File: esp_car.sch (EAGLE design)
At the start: 50 parts, among them IC2 LT1963ES8-3.3, SW2 SK-12D01, U1 ESP-WROOM-32_NOFLASH

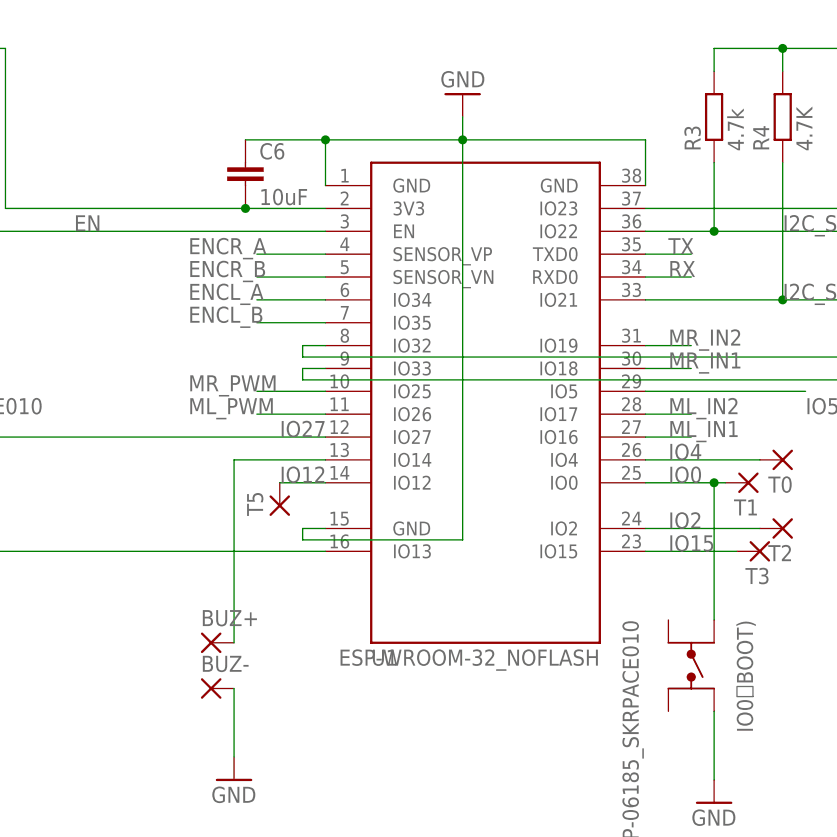
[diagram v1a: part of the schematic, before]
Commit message: wire 100% 初版
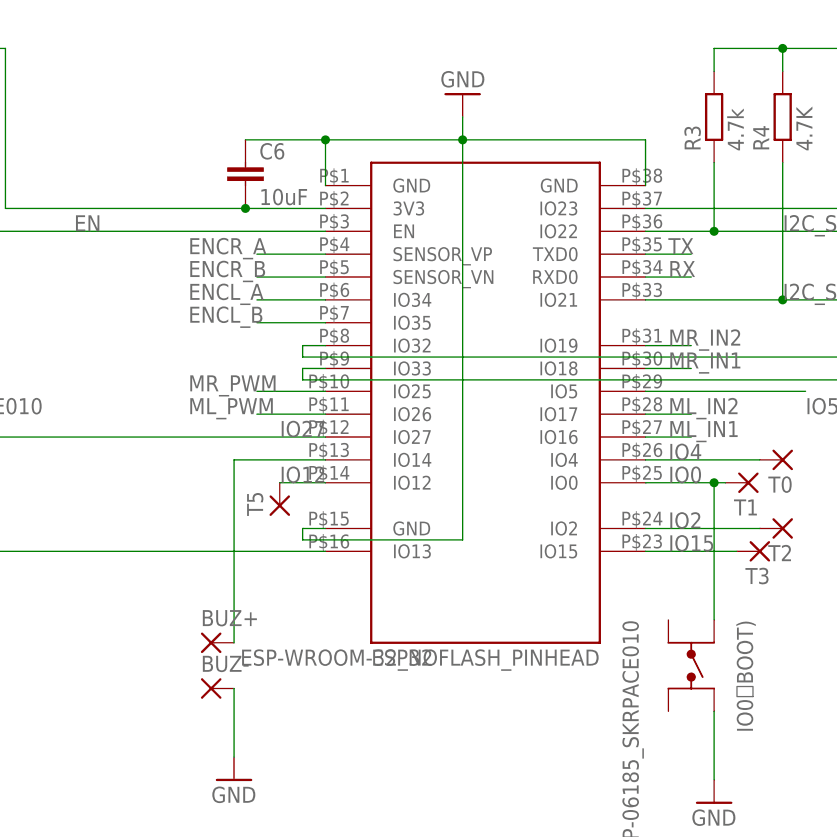
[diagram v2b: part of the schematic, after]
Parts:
- removed U1: ESP-WROOM-32_NOFLASH, esp32 _my:ESP-WROOM-32_NOFLASH
- added ESP32: ESP-WROOM-32_NOFLASH_PINHEAD, esp32 _my:ESP-WROOM-32_NOFLASH_PINHEAD
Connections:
- net +3V3: now also ESP32.3V3; no longer U1.3V3
- net EN: now also ESP32.EN; no longer U1.EN
- net ENCL_A: now also ESP32.IO34; no longer U1.IO34
- net ENCL_B: now also ESP32.IO35; no longer U1.IO35
- net ENCR_A: now also ESP32.SENSOR_VP; no longer U1.SENSOR_VP
- net ENCR_B: now also ESP32.SENSOR_VN; no longer U1.SENSOR_VN
- net GND: now also ESP32.GND@1, ESP32.GND@2, ESP32.GND@3; no longer U1.GND@1, U1.GND@2, U1.GND@3
- net I2C_SCL: now also ESP32.IO22; no longer U1.IO22
- net I2C_SDA: now also ESP32.IO21; no longer U1.IO21
- net IO0: now also ESP32.IO0; no longer U1.IO0
- net IO12: now also ESP32.IO12; no longer U1.IO12
- net IO15: now also ESP32.IO15; no longer U1.IO15
- net IO2: now also ESP32.IO2; no longer U1.IO2
- net IO27: now also ESP32.IO27; no longer U1.IO27
- net IO4: now also ESP32.IO4; no longer U1.IO4
- net IO5: now also ESP32.IO5; no longer U1.IO5
- net ML_IN1: now also ESP32.IO16; no longer U1.IO16
- net ML_IN2: now also ESP32.IO17; no longer U1.IO17
- net ML_PWM: now also ESP32.IO26; no longer U1.IO26
- net MR_IN1: now also ESP32.IO18; no longer U1.IO18
- net MR_IN2: now also ESP32.IO19; no longer U1.IO19
- net MR_PWM: now also ESP32.IO25; no longer U1.IO25
- net N$18: now also ESP32.IO13; no longer U1.IO13
- net N$19: now also ESP32.IO33; no longer U1.IO33
- net N$3: now also ESP32.IO32; no longer U1.IO32
- net N$5: now also ESP32.IO23; no longer U1.IO23
- net N$8: now also ESP32.IO14; no longer U1.IO14
- net RX: now also ESP32.RXD0; no longer U1.RXD0
- net TX: now also ESP32.TXD0; no longer U1.TXD0
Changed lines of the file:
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@@
 <?xml version="1.0" encoding="utf-8"?>
 <!DOCTYPE eagle SYSTEM "eagle.dtd">
-<eagle version="9.0.0">
+<eagle version="9.0.1">
 <drawing>
 <settings>
@@
 <clearance class="0" value="0.1524"/>
 </class>
-<class number="1" name="L" width="1.016" drill="0.4064">
+<class number="1" name="L" width="1.016" drill="0.8128">
 <clearance class="1" value="0.1524"/>
 </class>
@@
 <part name="GY-530C" library="pinhead" deviceset="PINHD-1X5" device=""/>
 <part name="GY-530L" library="pinhead" deviceset="PINHD-1X5" device=""/>
-<part name="U1" library="esp32 _my" deviceset="ESP-WROOM-32_NOFLASH" device=""/>
 <part name="U$1" library="adafruit_my" deviceset="TB6612_NEW" device=""/>
+<part name="ESP32" library="esp32 _my" deviceset="ESP-WROOM-32_NOFLASH_PINHEAD" device=""/>
 </parts>
 <sheets>
@@
 <instance part="GY-530C" gate="A" x="289.56" y="38.1"/>
 <instance part="GY-530L" gate="A" x="289.56" y="12.7"/>
-<instance part="U1" gate="G$1" x="172.72" y="83.82"/>
 <instance part="U$1" gate="G$1" x="398.78" y="60.96" rot="R180"/>
+<instance part="ESP32" gate="G$1" x="172.72" y="83.82"/>
 </instances>
 <busses>
@@
 <wire x1="170.18" y1="114.3" x2="190.5" y2="114.3" width="0.1524" layer="91"/>
 <wire x1="190.5" y1="114.3" x2="190.5" y2="109.22" width="0.1524" layer="91"/>
-<pinref part="U1" gate="G$1" pin="GND@1"/>
-<pinref part="U1" gate="G$1" pin="GND@3"/>
-<pinref part="U1" gate="G$1" pin="GND@2"/>
+<pinref part="ESP32" gate="G$1" pin="GND@1"/>
+<pinref part="ESP32" gate="G$1" pin="GND@3"/>
+<pinref part="ESP32" gate="G$1" pin="GND@2"/>
 </segment>
 <segment>
@@
 <junction x="146.05" y="106.68"/>
 <wire x1="154.94" y1="106.68" x2="146.05" y2="106.68" width="0.1524" layer="91"/>
-<pinref part="U1" gate="G$1" pin="3V3"/>
+<pinref part="ESP32" gate="G$1" pin="3V3"/>
 </segment>
 <segment>
@@
 <wire x1="114.3" y1="93.98" x2="109.22" y2="93.98" width="0.1524" layer="91"/>
 <label x="127" y="104.14" size="1.778" layer="95"/>
-<pinref part="U1" gate="G$1" pin="EN"/>
+<pinref part="ESP32" gate="G$1" pin="EN"/>
 </segment>
 </net>
@@
 <pinref part="T1" gate="1" pin="P"/>
 <wire x1="198.12" y1="76.2" x2="199.39" y2="76.2" width="0.1524" layer="91"/>
-<pinref part="U1" gate="G$1" pin="IO0"/>
+<pinref part="ESP32" gate="G$1" pin="IO0"/>
 </segment>
 </net>
@@
 <wire x1="190.5" y1="101.6" x2="195.58" y2="101.6" width="0.1524" layer="91"/>
 <label x="193.04" y="101.6" size="1.778" layer="95"/>
-<pinref part="U1" gate="G$1" pin="TXD0"/>
+<pinref part="ESP32" gate="G$1" pin="TXD0"/>
 </segment>
 <segment>
@@
 <wire x1="190.5" y1="99.06" x2="195.58" y2="99.06" width="0.1524" layer="91"/>
 <label x="193.04" y="99.06" size="1.778" layer="95"/>
-<pinref part="U1" gate="G$1" pin="RXD0"/>
+<pinref part="ESP32" gate="G$1" pin="RXD0"/>
 </segment>
 <segment>
@@
 <wire x1="154.94" y1="86.36" x2="147.32" y2="86.36" width="0.1524" layer="91"/>
 <label x="139.7" y="86.36" size="1.778" layer="95"/>
-<pinref part="U1" gate="G$1" pin="IO25"/>
+<pinref part="ESP32" gate="G$1" pin="IO25"/>
 </segment>
 </net>
@@
 <wire x1="190.5" y1="91.44" x2="195.58" y2="91.44" width="0.1524" layer="91"/>
 <label x="193.04" y="91.44" size="1.778" layer="95"/>
-<pinref part="U1" gate="G$1" pin="IO19"/>
+<pinref part="ESP32" gate="G$1" pin="IO19"/>
 </segment>
 </net>
@@
 <wire x1="190.5" y1="88.9" x2="195.58" y2="88.9" width="0.1524" layer="91"/>
 <label x="193.04" y="88.9" size="1.778" layer="95"/>
-<pinref part="U1" gate="G$1" pin="IO18"/>
+<pinref part="ESP32" gate="G$1" pin="IO18"/>
 </segment>
 </net>
@@
 <wire x1="190.5" y1="81.28" x2="195.58" y2="81.28" width="0.1524" layer="91"/>
 <label x="193.04" y="81.28" size="1.778" layer="95"/>
-<pinref part="U1" gate="G$1" pin="IO16"/>
+<pinref part="ESP32" gate="G$1" pin="IO16"/>
 </segment>
 </net>
@@
 <wire x1="190.5" y1="83.82" x2="195.58" y2="83.82" width="0.1524" layer="91"/>
 <label x="193.04" y="83.82" size="1.778" layer="95"/>
-<pinref part="U1" gate="G$1" pin="IO17"/>
+<pinref part="ESP32" gate="G$1" pin="IO17"/>
 </segment>
 </net>
@@
 <wire x1="154.94" y1="83.82" x2="147.32" y2="83.82" width="0.1524" layer="91"/>
 <label x="139.7" y="83.82" size="1.778" layer="95"/>
-<pinref part="U1" gate="G$1" pin="IO26"/>
+<pinref part="ESP32" gate="G$1" pin="IO26"/>
 </segment>
 </net>
@@
 <wire x1="154.94" y1="101.6" x2="147.32" y2="101.6" width="0.1524" layer="91"/>
 <label x="139.7" y="101.6" size="1.778" layer="95"/>
-<pinref part="U1" gate="G$1" pin="SENSOR_VP"/>
+<pinref part="ESP32" gate="G$1" pin="SENSOR_VP"/>
 </segment>
 </net>
@@
 <wire x1="154.94" y1="99.06" x2="147.32" y2="99.06" width="0.1524" layer="91"/>
 <label x="139.7" y="99.06" size="1.778" layer="95"/>
-<pinref part="U1" gate="G$1" pin="SENSOR_VN"/>
+<pinref part="ESP32" gate="G$1" pin="SENSOR_VN"/>
 </segment>
 </net>
@@
 <wire x1="154.94" y1="96.52" x2="147.32" y2="96.52" width="0.1524" layer="91"/>
 <label x="139.7" y="96.52" size="1.778" layer="95"/>
-<pinref part="U1" gate="G$1" pin="IO34"/>
+<pinref part="ESP32" gate="G$1" pin="IO34"/>
 </segment>
 </net>
@@
 <wire x1="154.94" y1="93.98" x2="147.32" y2="93.98" width="0.1524" layer="91"/>
 <label x="139.7" y="93.98" size="1.778" layer="95"/>
-<pinref part="U1" gate="G$1" pin="IO35"/>
+<pinref part="ESP32" gate="G$1" pin="IO35"/>
 </segment>
 </net>
@@
 <wire x1="149.86" y1="76.2" x2="154.94" y2="76.2" width="0.1524" layer="91"/>
 <label x="149.86" y="76.2" size="1.778" layer="95"/>
-<pinref part="U1" gate="G$1" pin="IO12"/>
+<pinref part="ESP32" gate="G$1" pin="IO12"/>
 </segment>
 <segment>
@@
 <pinref part="T0" gate="1" pin="P"/>
 <label x="193.04" y="78.74" size="1.778" layer="95"/>
-<pinref part="U1" gate="G$1" pin="IO4"/>
+<pinref part="ESP32" gate="G$1" pin="IO4"/>
 </segment>
 </net>
@@
 <pinref part="GY-530C" gate="A" pin="3"/>
 <pinref part="GY-530L" gate="A" pin="3"/>
-<pinref part="U1" gate="G$1" pin="IO22"/>
+<pinref part="ESP32" gate="G$1" pin="IO22"/>
 </segment>
 <segment>
@@
 <pinref part="GY-530C" gate="A" pin="4"/>
 <pinref part="GY-530L" gate="A" pin="4"/>
-<pinref part="U1" gate="G$1" pin="IO21"/>
+<pinref part="ESP32" gate="G$1" pin="IO21"/>
 </segment>
 <segment>
@@
 <wire x1="254" y1="106.68" x2="254" y2="58.42" width="0.1524" layer="91"/>
 <pinref part="GY-530R" gate="A" pin="5"/>
-<pinref part="U1" gate="G$1" pin="IO23"/>
+<pinref part="ESP32" gate="G$1" pin="IO23"/>
 </segment>
 </net>
@@
 <wire x1="190.5" y1="86.36" x2="208.28" y2="86.36" width="0.1524" layer="91"/>
 <label x="208.28" y="83.82" size="1.778" layer="95"/>
-<pinref part="U1" gate="G$1" pin="IO5"/>
+<pinref part="ESP32" gate="G$1" pin="IO5"/>
 </segment>
 <segment>
@@
 <wire x1="190.5" y1="71.12" x2="203.2" y2="71.12" width="0.1524" layer="91"/>
 <label x="193.04" y="71.12" size="1.778" layer="95"/>
-<pinref part="U1" gate="G$1" pin="IO2"/>
+<pinref part="ESP32" gate="G$1" pin="IO2"/>
 </segment>
 <segment>
@@
 <wire x1="190.5" y1="68.58" x2="200.66" y2="68.58" width="0.1524" layer="91"/>
 <label x="193.04" y="68.58" size="1.778" layer="95"/>
-<pinref part="U1" gate="G$1" pin="IO15"/>
+<pinref part="ESP32" gate="G$1" pin="IO15"/>
 </segment>
 <segment>
@@
 <pinref part="LED_FL" gate="G$1" pin="DI"/>
 <wire x1="109.22" y1="68.58" x2="109.22" y2="2.54" width="0.1524" layer="91"/>
-<pinref part="U1" gate="G$1" pin="IO13"/>
+<pinref part="ESP32" gate="G$1" pin="IO13"/>
 </segment>
 </net>
@@
 <wire x1="144.78" y1="78.74" x2="144.78" y2="58.42" width="0.1524" layer="91"/>
 <pinref part="BUZ+" gate="1" pin="P"/>
-<pinref part="U1" gate="G$1" pin="IO14"/>
+<pinref part="ESP32" gate="G$1" pin="IO14"/>
 </segment>
 </net>
@@
 <wire x1="251.46" y1="90.17" x2="251.46" y2="33.02" width="0.1524" layer="91"/>
 <pinref part="GY-530C" gate="A" pin="5"/>
-<pinref part="U1" gate="G$1" pin="IO32"/>
+<pinref part="ESP32" gate="G$1" pin="IO32"/>
 </segment>
 </net>
@@
 <wire x1="248.92" y1="87.63" x2="248.92" y2="7.62" width="0.1524" layer="91"/>
 <pinref part="GY-530L" gate="A" pin="5"/>
-<pinref part="U1" gate="G$1" pin="IO33"/>
+<pinref part="ESP32" gate="G$1" pin="IO33"/>
 </segment>
 </net>
@@
 <junction x="60.96" y="81.28"/>
 <wire x1="60.96" y1="81.28" x2="60.96" y2="78.74" width="0.1524" layer="91"/>
-<pinref part="U1" gate="G$1" pin="IO27"/>
-</segment>
-</net>
+<pinref part="ESP32" gate="G$1" pin="IO27"/>
+</segment>
+</net>
